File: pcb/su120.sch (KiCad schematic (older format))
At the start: 261 parts, among them J1 MJ-4PP-9, J2 Conn_01x03, J3 Conn_01x08, J4 Conn_01x08, J5 Conn_01x03, J6 MJ-4PP-9, SW1 SW_Push, SW10 SW_Push, SW11 SW_Push, SW12 SW_Push, SW13 SW_Push, SW14 SW_Push, SW15 SW_Push, SW16 SW_Push, SW17 SW_Push, SW18 SW_Push, SW19 SW_Push, SW2 SW_Push, SW20 SW_Push, SW3 SW_Push, SW4 SW_Push, SW5 SW_Push, SW6 SW_Push, SW7 SW_Push, SW8 SW_Push, SW9 SW_Push, U1 ProMicro

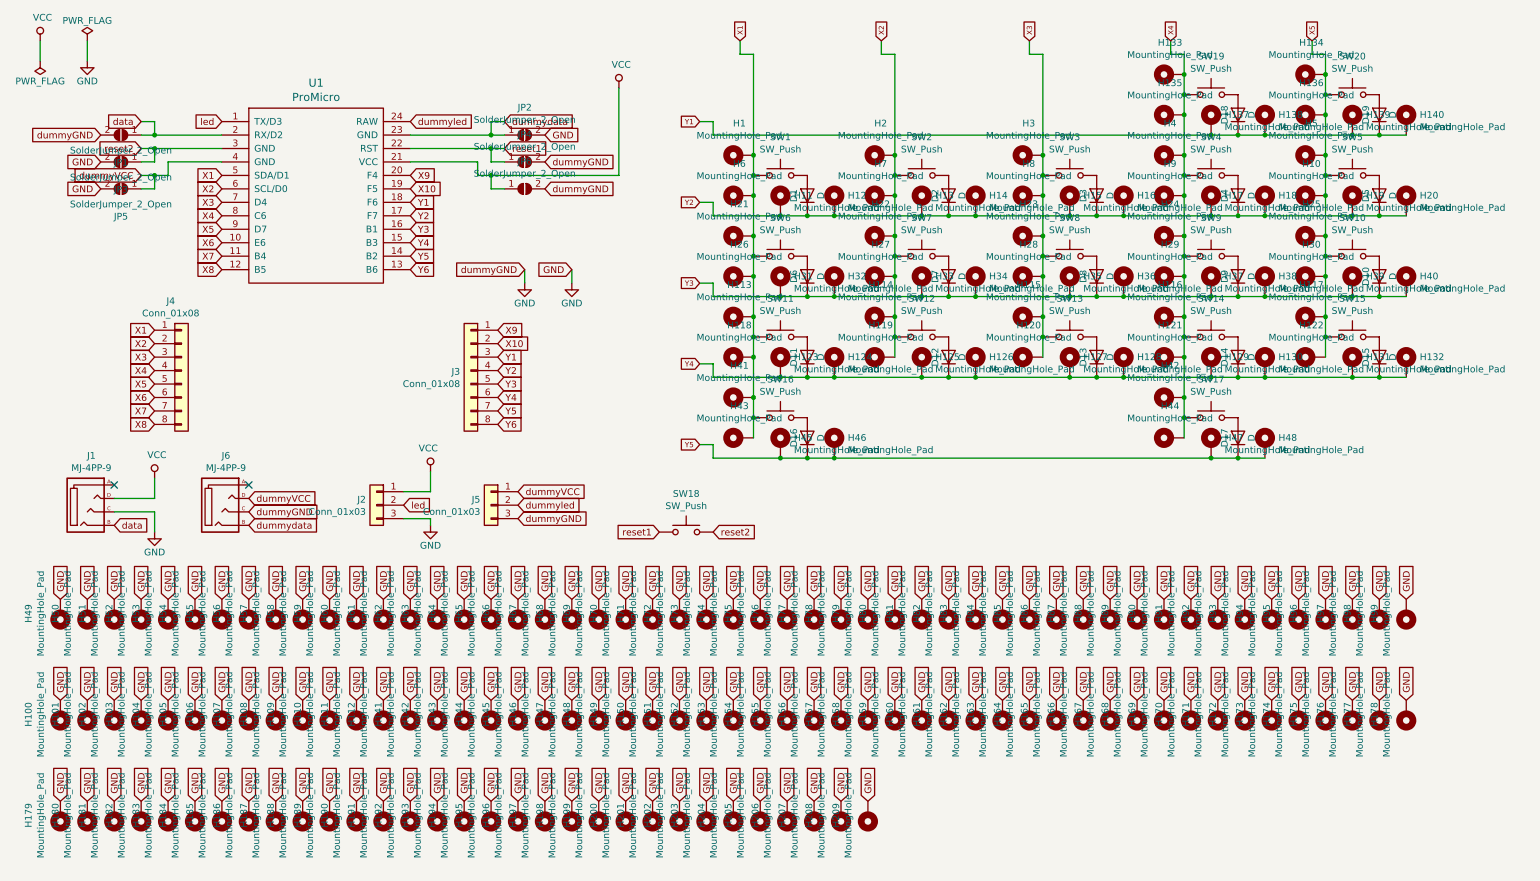
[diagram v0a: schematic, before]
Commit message: Rev.3
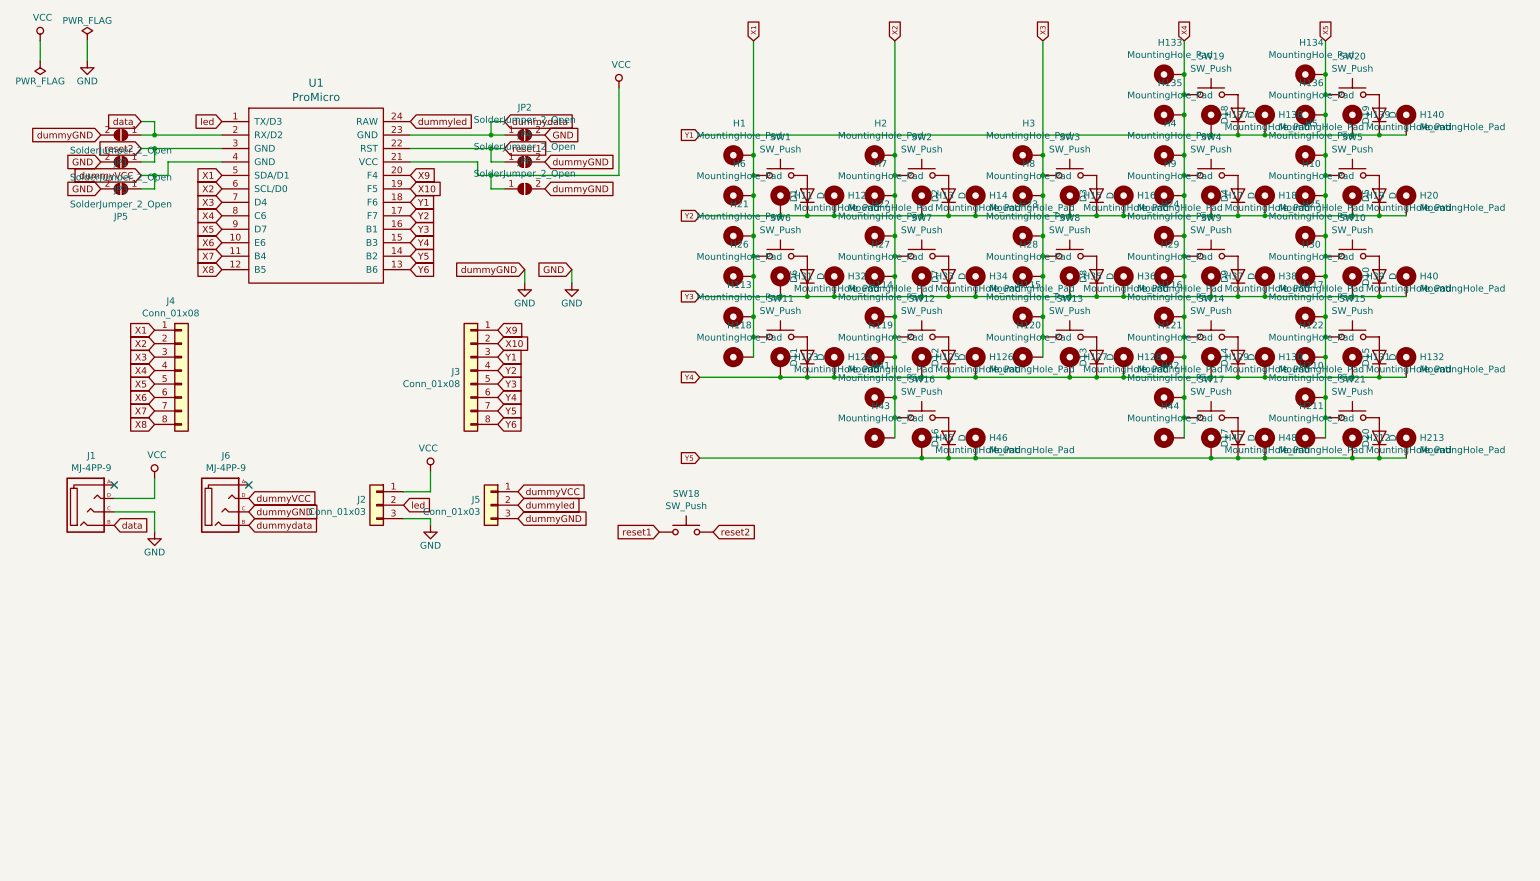
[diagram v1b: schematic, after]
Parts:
- removed H100, H101, H102, H103, H104, H105, H106, H107, H108, H109, H110, H111, H112, H141, H142, H143, H144, H145, H146, H147, H148, H149, H150, H151, H152, H49, H50, H51, H52, H53, H54, H55, H56, H57, H58, H59, H60, H61, H62, H63, H64, H65, H66, H67, H68, H69, H70, H71, H72, H73, H74, H75, H76, H77, H78, H79, H80, H81, H82, H83, H84, H85, H86, H87, H88, H89, H90, H91, H92, H93, H94, H95, H96, H97, H98, H99: MountingHole_Pad, #footprint:M2_Pad, symbol Mechanical:MountingHole_Pad
- removed H153, H154, H155, H156, H157, H158, H159, H160, H161, H162, H163, H164, H165, H166, H167, H168, H169, H170, H171, H172, H173, H174, H175, H176, H177, H178, H179, H180, H181, H182, H183, H184, H185, H186, H187, H188, H189, H190, H191, H192, H193, H194, H195, H196, H197, H198, H199, H200, H201, H202, H203, H204, H205, H206, H207, H208, H209: MountingHole_Pad, #footprint:M1.4_tapping_Pad, symbol Mechanical:MountingHole_Pad
- added D20: D, #footprint:diode_TH_SMD, symbol Device:D
- added H210, H211, H212, H213: MountingHole_Pad, #footprint:1pin_conn, symbol Mechanical:MountingHole_Pad
- added SW21: SW_Push, #footprint:CherryMX_MidHeight_Choc_Hotswap_rev4, symbol Switch:SW_Push
- SW1, SW10, SW11, SW12, SW13, SW14, SW15, SW16, SW17, SW19, SW2, SW20, SW3, SW4, SW5, SW6, SW7, SW8, SW9: footprint #footprint:CherryMX_MidHeight_Choc_Hotswap_rev2 -> #footprint:CherryMX_MidHeight_Choc_Hotswap_rev4
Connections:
- net X1: no longer H41.1, H43.1, SW16.1
- net X2: now also H41.1, H43.1, SW16.1
- net X5: now also H210.1, H211.1, SW21.1
- net Y5: now also D20.1 (K), H212.1, H213.1
- new net: D20.2 (A), SW21.2
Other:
- moved on the sheet: D16, H41, H43, H45, H46, SW16

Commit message: Rev.4
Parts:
- J3, J4: footprint #footprint:PinHeader_1x08_P2.54mm_Vertical -> #footprint:PinHeader_1x08_P2.54mm_Vertical_rev2
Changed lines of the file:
@@
 F 0 "J3" H 3980 3242 50  0000 L CNN
 F 1 "Conn_01x08" H 3980 3151 50  0000 L CNN
-F 2 "#footprint:PinHeader_1x08_P2.54mm_Vertical" H 3900 3250 50  0001 C CNN
+F 2 "#footprint:PinHeader_1x08_P2.54mm_Vertical_rev2" H 3900 3250 50  0001 C CNN
 F 3 "~" H 3900 3250 50  0001 C CNN
 	1    3900 3250
@@
 F 0 "J4" H 1670 3767 50  0000 C CNN
 F 1 "Conn_01x08" H 1670 3676 50  0000 C CNN
-F 2 "#footprint:PinHeader_1x08_P2.54mm_Vertical" H 1750 3250 50  0001 C CNN
+F 2 "#footprint:PinHeader_1x08_P2.54mm_Vertical_rev2" H 1750 3250 50  0001 C CNN
 F 3 "~" H 1750 3250 50  0001 C CNN
 	1    1750 3250
